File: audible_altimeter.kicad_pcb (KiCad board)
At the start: 2 copper layers, 80 x 45 mm, 87 parts, among them CON1 BUQ2-USB-MICRO-B, IC1 BUQ2-ATXMEGA128A4U-A, P1 CONN_2, Q1 NPN, SW1 SW_LEFT, SW2 SW_DOWN, SW3 SW_UP, SW4 SW_CENTER, SW5 SW_RIGHT, U1 MCP7940M, U10 MPU-9250, U11 SIM33ELA, U12 SI7020-A10, U13 FLASH_MEMORY, U14 RAM_MEMORY, U2 MCP73831-SOT-23-5, U3 NCP4681-SC-70, U4 MICRO-SD-CONN, U5 MPL3115A2, U6 MS5805-02BA01, U7 LS013B4DN04, U8 CSS-0575A-SMT, U9 TAG-CONNECT-ATMEL-PDI-CONNECT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, X1 CRYSTAL

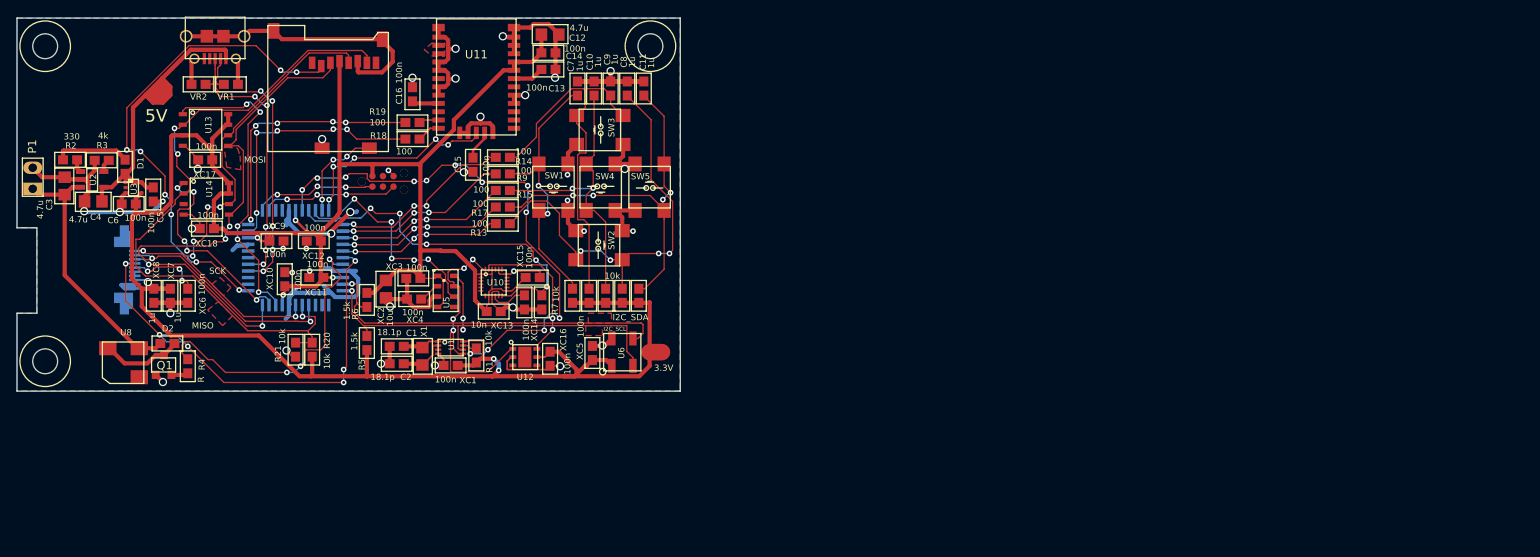
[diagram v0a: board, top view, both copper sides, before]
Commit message: Start planning test board v2.0
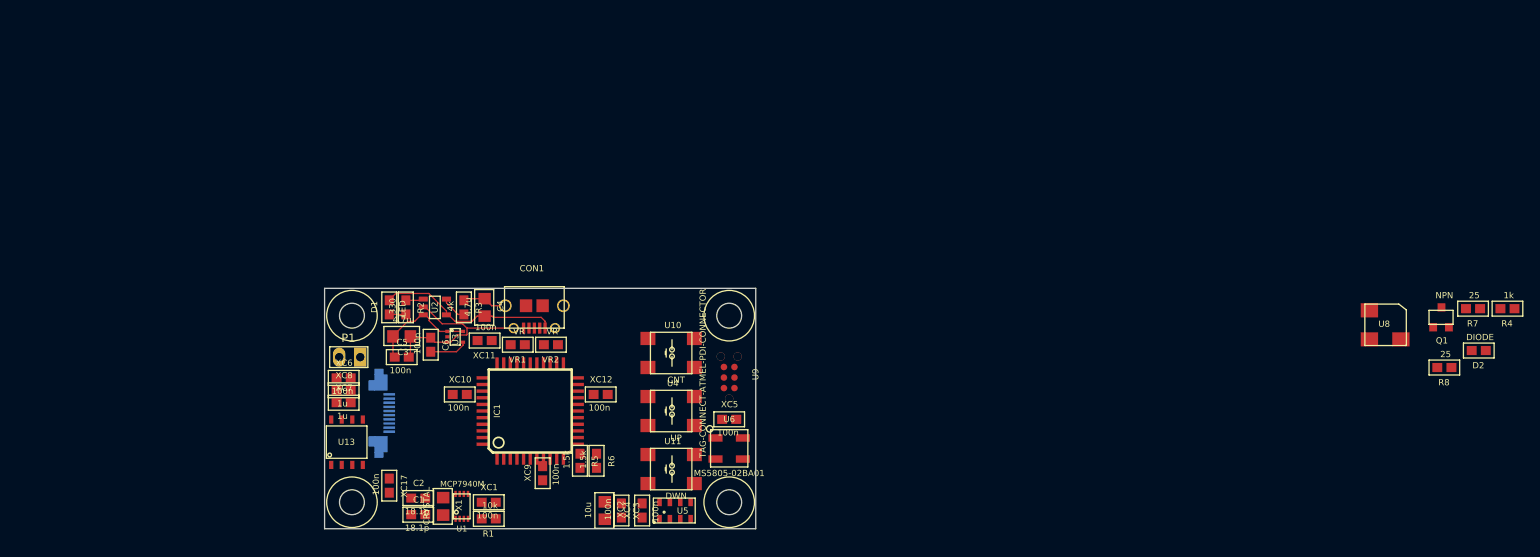
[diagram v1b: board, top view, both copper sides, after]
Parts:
- removed C10, C11, C7, C8, C9: 1u, buq2:SM0603
- removed C12: 4.7u, buq2:SM0805
- removed C13, C14, C15, C16, XC14, XC15, XC16, XC18: 100n, buq2:SM0603
- removed LS013B4DN04-FPC: VAL**, buq2:LS013B4DN04-FPC
- removed the MOUNTING_HOLE at (102.0, 67.0)
- removed the MOUNTING_HOLE at (102.0, 105.0)
- removed the MOUNTING_HOLE at (175.0, 67.0)
- removed R10, R11, R12, R16, R20, R21: 10k, buq2:SM0603
- removed R13, R14, R15, R17, R18, R19, R9: 100, buq2:SM0603
- removed SW1: SW_LEFT, buq2:PUSHBUTTON_4x4_5x5_ROTATED
- removed SW2: SW_DOWN, buq2:PUSHBUTTON_4x4_5x5_ROTATED
- removed SW3: SW_UP, buq2:PUSHBUTTON_4x4_5x5_ROTATED
- removed SW4: SW_CENTER, buq2:PUSHBUTTON_4x4_5x5_ROTATED
- removed SW5: SW_RIGHT, buq2:PUSHBUTTON_4x4_5x5_ROTATED
- removed U12: SI7020-A10, buq2:DFN-6-3X3MM
- removed U14: RAM_MEMORY, buq2:8-SOIC
- removed XC13: 10n, buq2:SM0603
- added MOUNTING_HOLE: VAL**, buq2:MOUNTING_HOLE, F.Cu at (139.0, 122.0)
- added MOUNTING_HOLE: VAL**, buq2:MOUNTING_HOLE, F.Cu at (184.5, 122.0)
- added MOUNTING_HOLE: VAL**, buq2:MOUNTING_HOLE, F.Cu at (184.5, 99.5)
- added MOUNTING_HOLE: VAL**, buq2:MOUNTING_HOLE, F.Cu at (139.0, 99.5)
- IC1: moved to F.Cu
- R4: value R -> 1k
- R7, R8: value 10k -> 25
- U10: value MPU-9250 -> CNT; footprint buq2:24QFN-3MM-3MM -> buq2:PUSHBUTTON_4x4_5x5_ROTATED_4_PIN
- U11: value SIM33ELA -> DWN; footprint buq2:SIM33ELA-GPS -> buq2:PUSHBUTTON_4x4_5x5_ROTATED_4_PIN
- U4: value MICRO-SD-CONN -> UP; footprint buq2:MICRO-SD-CONN-AMPHENOL-PUSH-PUSH -> buq2:PUSHBUTTON_4x4_5x5_ROTATED_4_PIN
- U7: footprint buq2:FPC-CONN-10-FCI-BOTTOM-CONTACTS -> buq2:FPC-CONN-10-FCI-TOP-CONTACTS
- moved R4 159.3 mm to (278.4, 98.7), turned to 0 degrees
- moved D2 158.2 mm to (274.9, 103.7), turned to 0 degrees
- moved Q1 154.2 mm to (270.4, 99.7)
- moved U8 148.4 mm to (261.7, 102.4), turned to 0 degrees
- moved R7 112.3 mm to (274.2, 98.7), turned to 0 degrees
- moved R8 105.5 mm to (270.8, 105.8), turned to 0 degrees
- moved VR2 52.8 mm to (163.0, 103.0), turned to 0 degrees
- moved U11 52.6 mm to (177.5, 118.0), turned to 0 degrees
- moved U4 51.9 mm to (177.5, 111.0)
- moved U9 51.5 mm to (184.5, 109.5), turned to 90 degrees
- moved CON1 50.4 mm to (161.0, 101.0)
- moved C4 48.9 mm to (155.0, 98.5), turned to 90 degrees
- moved R3 47.1 mm to (152.5, 98.5), turned to 90 degrees
- moved VR1 46.7 mm to (159.0, 103.0), turned to 0 degrees
- moved U13 45.9 mm to (136.5, 117.5), turned to 0 degrees
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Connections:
- C5 pad 2: /Battery/+5V -> /Battery/BATTERY
- IC1 pad 10: /9-Axis/I2C_SDA -> /Barometer/I2C_SDA
- IC1 pad 11: /9-Axis/I2C_SCL -> /Barometer/I2C_SCL
- IC1 pad 2: /Buttons/BUTTON_LEFT -> /Buttons/BUTTON_CENTER
- IC1 pad 21: /MCU/CSn_RAM -> /Display/CS
- IC1 pad 22: /Display/CS -> /Display/DISP_ON
- IC1 pad 23: /MicroSD/CSn -> (no net)
- IC1 pad 24: (no net) -> /Buzzer/BUZZER_DRIVE
- IC1 pad 3: /Buttons/BUTTON_CENTER -> /Buttons/BUTTON_DOWN
- IC1 pad 32: /GPS/RX -> (no net)
- IC1 pad 33: /GPS/TX -> (no net)
- IC1 pad 4: /Buttons/BUTTON_RIGHT -> (no net)
- IC1 pad 41: /MCU/ACCELERATOR_INT -> (no net)
- IC1 pad 43: /MicroSD/CARD_DETECT -> (no net)
- IC1 pad 44: /MCU/GPS_PULSE_PER_SECOND -> (no net)
- IC1 pad 5: /Buttons/BUTTON_DOWN -> (no net)
- IC1 pad 6: /MCU/DISPLAY_INVERT -> (no net)
- IC1 pad 7: /Buzzer/BUZZER_DRIVE -> (no net)
- R5 pad 2: /9-Axis/I2C_SCL -> /Barometer/I2C_SCL
- R6 pad 2: /9-Axis/I2C_SDA -> /Barometer/I2C_SDA
- R7 pad 1: GND -> Net-(R7-Pad1)
- R7 pad 2: /MCU/ACCELERATOR_INT -> /Battery/BATTERY
- R8 pad 1: /Battery/+3.3V -> Net-(R8-Pad1)
- R8 pad 2: Net-(C7-Pad1) -> Net-(R7-Pad1)
- U1 pad 5: /9-Axis/I2C_SDA -> /Barometer/I2C_SDA
- U1 pad 6: /9-Axis/I2C_SCL -> /Barometer/I2C_SCL
- U10 pad 1: /Battery/+3.3V -> GND
- U10 pad 4: (no net) -> /Buttons/BUTTON_CENTER
- U11 pad 1: (no net) -> GND
- U11 pad 4: GND -> /Buttons/BUTTON_DOWN
- U3 pad 1: /Battery/+5V -> /Battery/BATTERY
- U3 pad 5: /Battery/+5V -> /Battery/BATTERY
- U4 pad 1: (no net) -> GND
- U4 pad 2: /MicroSD/CSn -> (no net)
- U4 pad 3: /Display/MOSI -> (no net)
- U4 pad 4: /Battery/+3.3V -> /Buttons/BUTTON_UP
- U5 pad 7: /9-Axis/I2C_SDA -> /Barometer/I2C_SDA
- U5 pad 8: /9-Axis/I2C_SCL -> /Barometer/I2C_SCL
- U6 pad 2: /9-Axis/I2C_SCL -> /Barometer/I2C_SCL
- U6 pad 3: /9-Axis/I2C_SDA -> /Barometer/I2C_SDA
- U7 pad 4: /MCU/DISPLAY_INVERT -> GND
- U7 pad 8: /Battery/+3.3V -> GND
- U8 pad 1: /Battery/BATTERY -> Net-(R8-Pad1)
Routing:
- net /Battery/+3.3V: track 333.2 -> 4.58 mm, vias 7 -> 0
- net GND: track 271.0 -> 28.3 mm, vias 39 -> 0
- net /MCU/MISO: track 81.7 -> 0.00 mm, vias 3 -> 0
- net /9-Axis/I2C_SDA: track 76.8 -> 0.00 mm, vias 5 -> 0
- net /9-Axis/I2C_SCL: track 73.8 -> 0.00 mm, vias 5 -> 0
- net /Display/MOSI: track 72.0 -> 0.00 mm, vias 4 -> 0
- net /MCU/CLOCK_INT: track 67.3 -> 0.00 mm, vias 13 -> 0
- net /MCU/SCK: track 64.7 -> 0.00 mm, vias 6 -> 0
- net /MicroSD/CSn: track 59.4 -> 0.00 mm, vias 8 -> 0
- net /MCU/DISPLAY_INVERT: track 56.7 -> 0.00 mm, vias 6 -> 0
- net Net-(C8-Pad1): track 52.0 -> 0.00 mm, vias 4 -> 0
- net /Battery/+5V: track 72.3 -> 22.2 mm
- net Net-(C9-Pad1): track 46.9 -> 0.00 mm
- net Net-(C11-Pad1): track 46.8 -> 0.00 mm, vias 4 -> 0
- net /MCU/ACCELERATOR_INT: track 45.1 -> 0.00 mm, vias 5 -> 0
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- removed copper zone on F.Cu, net /9-Axis/I2C_SCL
- removed copper zone on F.Cu, net /9-Axis/I2C_SDA
- removed copper zone on F.Cu, net /Display/MOSI
- removed copper zone on F.Cu, net /MCU/MISO
- removed copper zone on F.Cu, net /MCU/SCK
- removed copper zone on B.Cu, net GND
- removed copper zone on F.Cu, net Net-(U11-Pad16)
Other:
- board size 80 x 45 mm -> 52 x 29 mm
- board text removed: "3.3V"
- board text removed: "5V"
- board text removed: "AudibleA V1.0"
- board text removed: "I2C_SCL"
- board text removed: "I2C_SDA"
- board text removed: "MISO"
- board text removed: "MOSI"
- board text removed: "SCK"

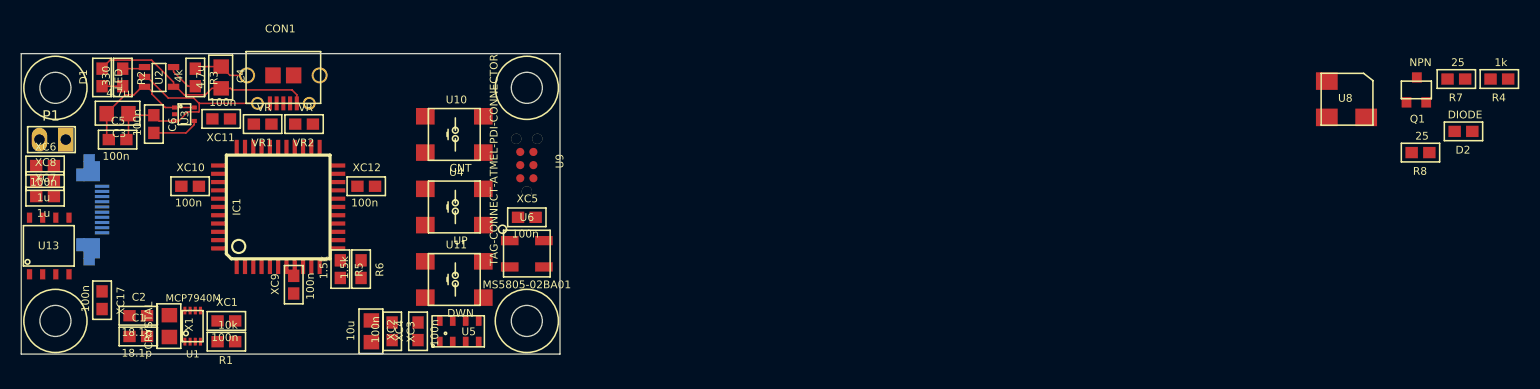
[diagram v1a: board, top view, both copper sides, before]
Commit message: Almost ready routing
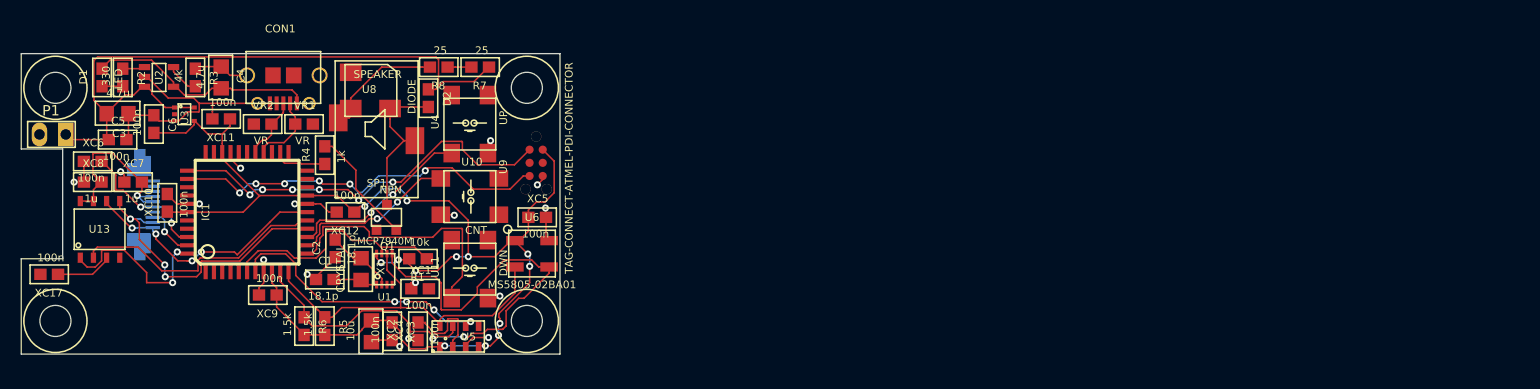
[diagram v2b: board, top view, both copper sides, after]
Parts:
- added LS013B7DH03-FPC: VAL**, buq2:LS013B7DH03-FPC, F.Cu at (138.8, 142.5)
- added SP1: SPEAKER, buq2:SPEAKER_240326000031, F.Cu at (170.0, 103.5)
- moved R4 113.6 mm to (165.0, 106.0), turned to 270 degrees
- moved Q1 100.2 mm to (171.0, 112.0)
- moved D2 100.0 mm to (175.0, 100.5), turned to 90 degrees
- moved R8 95.1 mm to (176.0, 97.5)
- moved R7 94.2 mm to (180.0, 97.5)
- moved U8 94.2 mm to (167.5, 101.5)
- moved R1 20.2 mm to (174.0, 116.0)
- moved C2 20.1 mm to (166.0, 115.0), turned to 270 degrees
- moved U1 19.3 mm to (170.0, 118.5)
- moved X1 19.3 mm to (168.5, 117.0)
- moved XC1 19.0 mm to (174.2, 118.9)
- moved C1 18.8 mm to (165.0, 118.0)
- moved XC7 8.61 mm to (146.5, 108.6)
- moved U4 8.14 mm to (179.0, 103.0), turned to 90 degrees
- moved R6 7.78 mm to (163.0, 122.5)
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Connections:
- IC1 pad 1: /Buttons/BUTTON_UP -> (no net)
- IC1 pad 12: (no net) -> /Buttons/BUTTON_DOWN
- IC1 pad 13: (no net) -> /Buttons/BUTTON_CENTER
- IC1 pad 14: (no net) -> /Buttons/BUTTON_UP
- IC1 pad 2: /Buttons/BUTTON_CENTER -> (no net)
- IC1 pad 20: /MCU/CSn_FLASH -> (no net)
- IC1 pad 21: /Display/CS -> (no net)
- IC1 pad 22: /Display/DISP_ON -> (no net)
- IC1 pad 3: /Buttons/BUTTON_DOWN -> (no net)
- IC1 pad 40: /MCU/CLOCK_INT -> (no net)
- IC1 pad 42: /MCU/BAROMETER_INT -> /Display/DISP_ON
- IC1 pad 43: (no net) -> /Display/CS
- IC1 pad 44: (no net) -> /MCU/CSn_FLASH
- IC1 pad 6: (no net) -> /MCU/CLOCK_INT
- IC1 pad 7: (no net) -> /MCU/BAROMETER_INT
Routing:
- net /Battery/+3.3V: track 4.58 -> 145.9 mm, vias 0 -> 15
- net /Barometer/I2C_SDA: track 0.00 -> 61.7 mm, vias 0 -> 2
- net /Battery/BATTERY: track 13.1 -> 66.3 mm
- net GND: track 28.3 -> 67.3 mm, vias 0 -> 15
- net /MCU/PDI_DATA: track 0.00 -> 38.9 mm, vias 0 -> 6
- net /MCU/PDI_CLK: track 0.00 -> 36.8 mm, vias 0 -> 6
- net /Barometer/I2C_SCL: track 0.00 -> 35.5 mm
- net /Display/MOSI: track 0.00 -> 28.1 mm, vias 0 -> 3
- net /MCU/BAROMETER_INT: track 0.00 -> 26.2 mm, vias 0 -> 4
- net /Buttons/BUTTON_DOWN: track 0.00 -> 25.3 mm
- net /MCU/MISO: track 0.00 -> 25.2 mm
- net /MCU/SCK: track 0.00 -> 24.5 mm, vias 0 -> 4
- net /MCU/CLOCK_INT: track 0.00 -> 22.7 mm
- net /Buttons/BUTTON_UP: track 0.00 -> 17.9 mm, vias 0 -> 2
- net /Buttons/BUTTON_CENTER: track 0.00 -> 16.9 mm, vias 0 -> 2
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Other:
- outline, holes or cut-outs redrawn
